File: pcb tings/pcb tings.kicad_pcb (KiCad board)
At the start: 2 copper layers, 77 x 38.1 mm, 24 parts, among them SW1 SW_Push, U1 ATmega32U4-A, Y1 16MHz

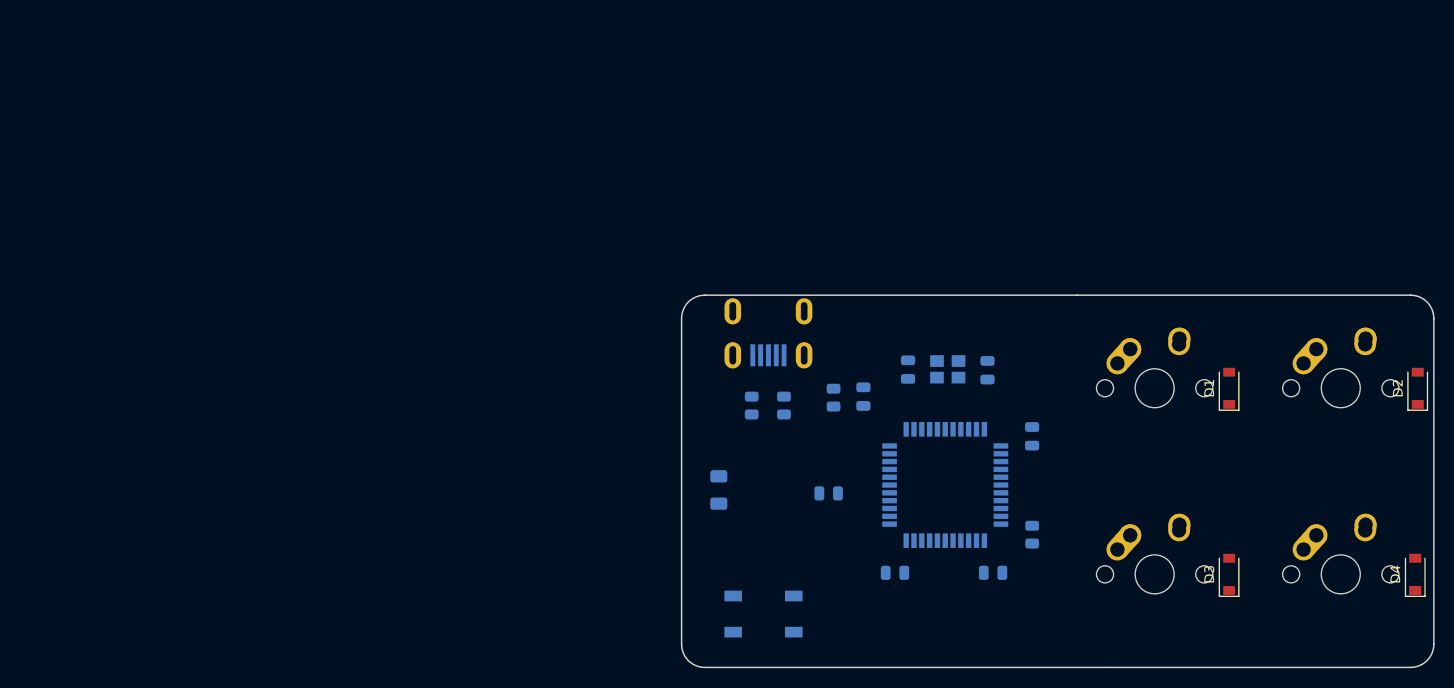
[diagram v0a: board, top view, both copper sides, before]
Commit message: Routing
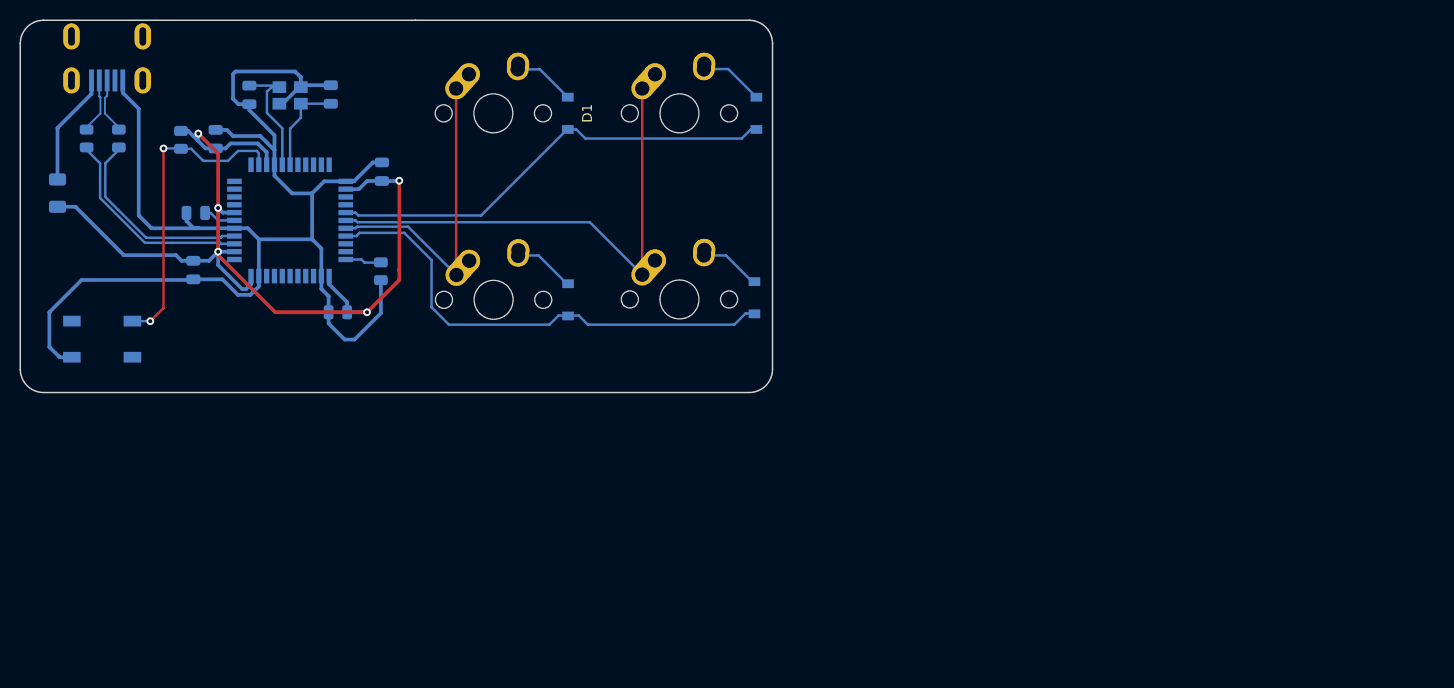
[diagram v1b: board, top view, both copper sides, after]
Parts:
- D1, D2, D3, D4: moved to B.Cu
- moved C7 78.2 mm to (62.7, 87.1), turned to -90 degrees
- moved F1 74.2 mm to (48.8, 79.2)
- moved R2 73.4 mm to (55.1, 73.7)
- moved R3 73.4 mm to (51.8, 73.7)
- moved D4 73.3 mm to (120.2, 90.0)
- moved USB1 73.3 mm to (53.9, 63.2)
- moved D1 73.3 mm to (101.1, 71.1)
- moved D2 73.3 mm to (120.4, 71.1)
- moved MX1 73.3 mm to (93.4, 71.1)
- moved MX2 73.3 mm to (112.5, 71.1)
- moved MX4 73.3 mm to (112.5, 90.1)
- moved SW1 73.3 mm to (53.4, 94.2)
- moved D3 73.3 mm to (101.1, 90.2)
- moved MX3 73.3 mm to (93.5, 90.2)
- moved C2 73.0 mm to (68.5, 69.2)
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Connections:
- net Net-(USB1-Pad3) renamed D+
- net Net-(USB1-Pad4) renamed D-
- C1 pad 2: GND -> +5V
- C2 pad 2: GND -> +5V
- C3 pad 2: GND -> +5V
- C4 pad 2: GND -> +5V
- C5 pad 2: GND -> +5V
- C6 pad 2: GND -> +5V
- C7 pad 2: GND -> +5V
- D1 pad 1: Net-(D1-Pad1) -> ROW0
- D2 pad 1: Net-(D1-Pad1) -> ROW0
- D3 pad 1: Net-(D3-Pad1) -> ROW1
- D4 pad 1: Net-(D3-Pad1) -> ROW1
- R4 pad 1: GND -> +5V
- SW1 pad 1: GND -> +5V
- U1 pad 15: GND -> +5V
- U1 pad 23: GND -> +5V
- U1 pad 35: GND -> +5V
- U1 pad 43: GND -> +5V
- U1 pad 5: GND -> +5V
- USB1 pad 1: GND -> +5V
- Y1 pad 2: GND -> +5V
- Y1 pad 4: GND -> +5V
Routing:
- net +5V: track 0.00 -> 241.4 mm, vias 0 -> 5
- net COL1: track 0.00 -> 51.7 mm
- net ROW1: track 0.00 -> 49.9 mm
- net ROW0: track 0.00 -> 46.6 mm
- net COL0: track 0.00 -> 32.4 mm
- net Net-(R1-Pad2): track 0.00 -> 32.0 mm, vias 0 -> 2
- net Net-(U1-Pad3): track 0.00 -> 21.4 mm
- net Net-(U1-Pad4): track 0.00 -> 20.6 mm
- net Net-(U1-Pad16): track 0.00 -> 12.7 mm
- net VCC: track 0.00 -> 11.6 mm
- net Net-(U1-Pad17): track 0.00 -> 9.76 mm
- net Net-(D2-Pad2): track 0.00 -> 6.58 mm
- net Net-(D3-Pad2): track 0.00 -> 6.30 mm
- net Net-(D1-Pad2): track 0.00 -> 6.30 mm
- net Net-(D4-Pad2): track 0.00 -> 6.30 mm
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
